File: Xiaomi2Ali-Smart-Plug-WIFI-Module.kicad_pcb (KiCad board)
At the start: 2 copper layers, 18.6 x 45 mm, 9 parts, among them J1 Conn_01x07, J2 Conn_01x03, SW1 SW_Push

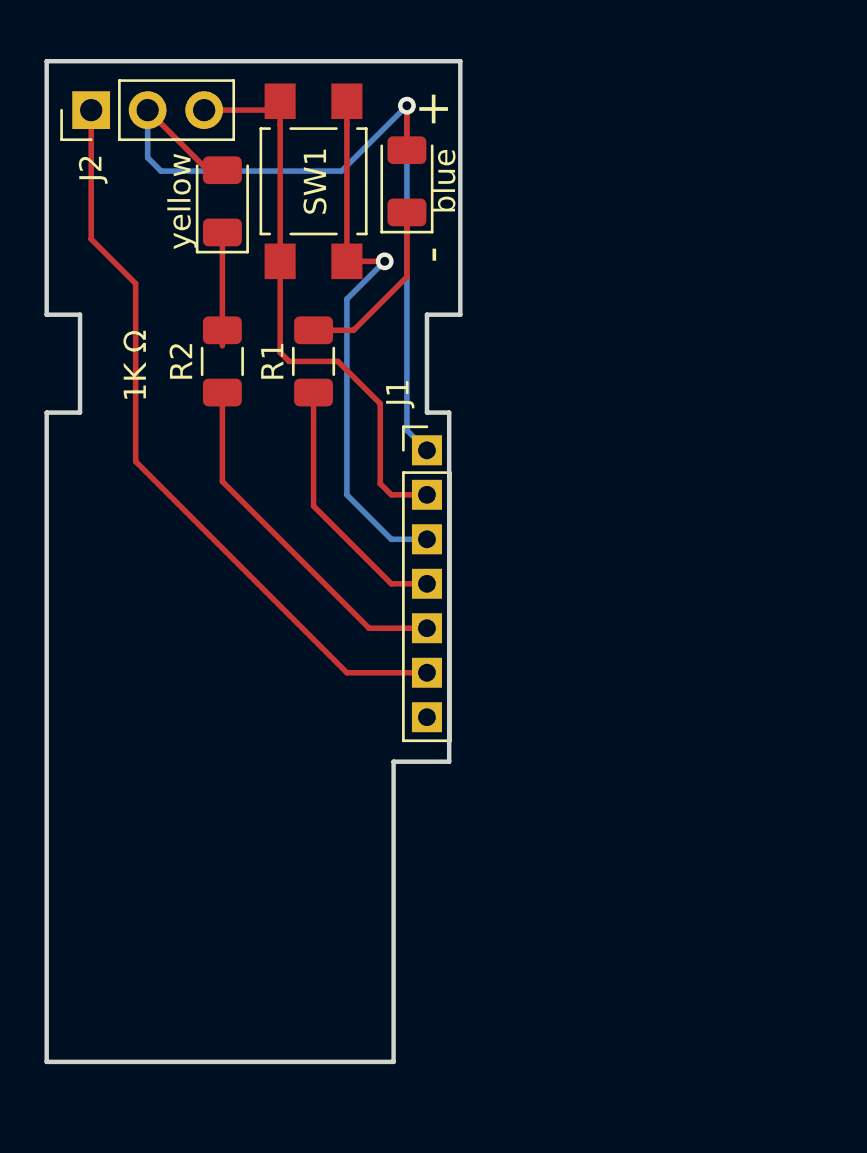
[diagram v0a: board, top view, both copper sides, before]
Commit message: Updated: 2019-02-18 18:36:52
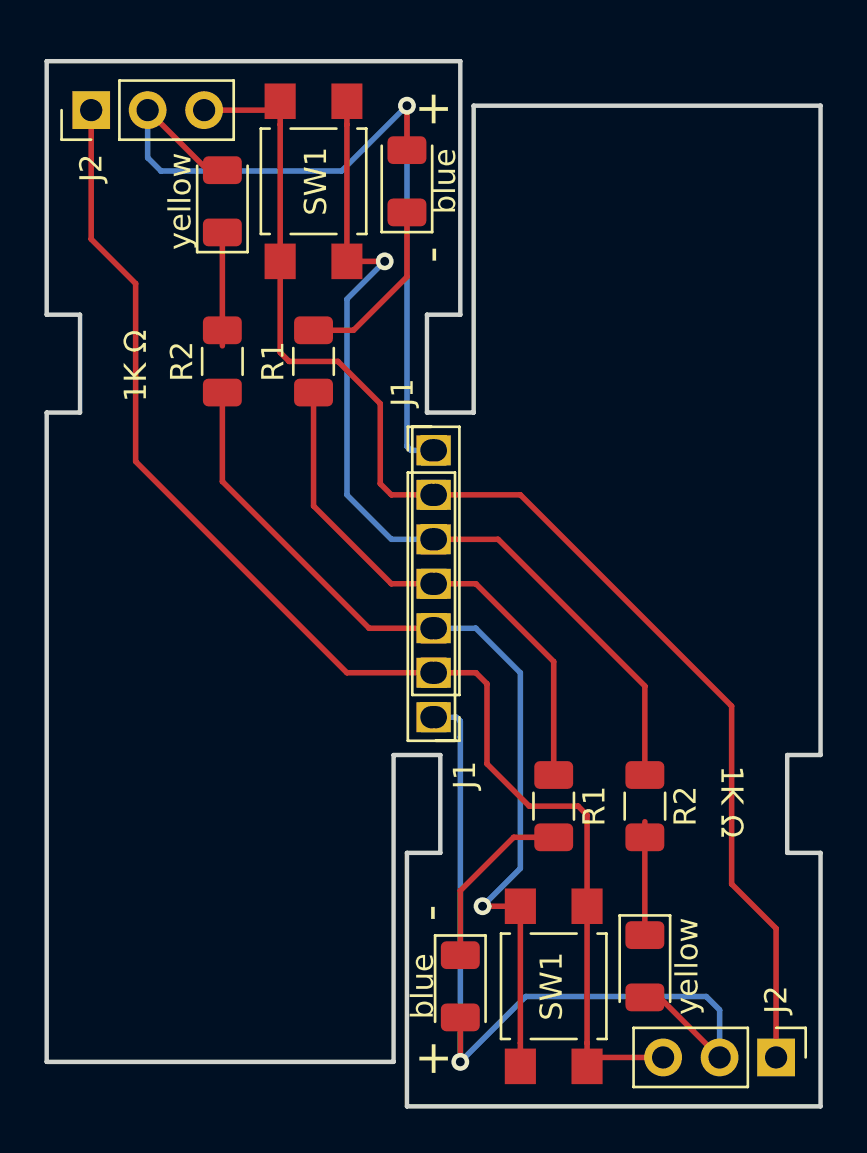
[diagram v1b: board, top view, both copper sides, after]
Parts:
- removed the J1 at (143.1, 87.5)
- added J1: Conn_01x07, Connector_PinHeader_2.00mm:PinHeader_1x07_P2.00mm_Vertical, F.Cu at (143.3, 87.5)
- added J1: Conn_01x07, Connector_PinHeader_2.00mm:PinHeader_1x07_P2.00mm_Vertical, F.Cu at (143.5, 99.5)
- added J2: Conn_01x03, Connector_PinHeader_2.54mm:PinHeader_1x03_P2.54mm_Vertical, F.Cu at (158.8, 114.8)
- added R1: 1K, Resistor_SMD:R_1206_3216Metric, F.Cu at (148.8, 103.5)
- added R2: 1K, Resistor_SMD:R_1206_3216Metric, F.Cu at (152.9, 103.5)
- added REF**: OSHW-Logo2_9.8x8mm_SilkScreen, Symbol:OSHW-Logo2_9.8x8mm_SilkScreen, B.Cu at (152.8, 86.2)
- added REF**: KiCad-Logo2_6mm_SilkScreen, Symbol:KiCad-Logo2_6mm_SilkScreen, B.Cu at (152.8, 77.0)
- added SW1: SW_Push, Button_Switch_SMD:SW_SPST_TL3305A, F.Cu at (148.8, 111.6)
- added blue: LED_blue, LED_SMD:LED_1206_3216Metric, F.Cu at (144.6, 111.6)
- added yellow: LED_yellow, LED_SMD:LED_1206_3216Metric, F.Cu at (152.9, 110.7)
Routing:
- net (no net): track 0.00 -> 163.9 mm, vias 0 -> 2
- net VCC: track 37.0 -> 38.2 mm
- net Net-(J1-Pad6): track 33.2 -> 33.9 mm
- net Net-(J1-Pad5): track 15.5 -> 16.1 mm
- net Net-(J1-Pad4): track 11.2 -> 11.8 mm
- net Net-(J1-Pad3): track 24.3 -> 24.9 mm
- net GND: track 25.8 -> 26.4 mm
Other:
- board size 18.6 x 45 mm -> 34.8 x 47 mm

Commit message: Updated: 2019-02-20 00:25:07
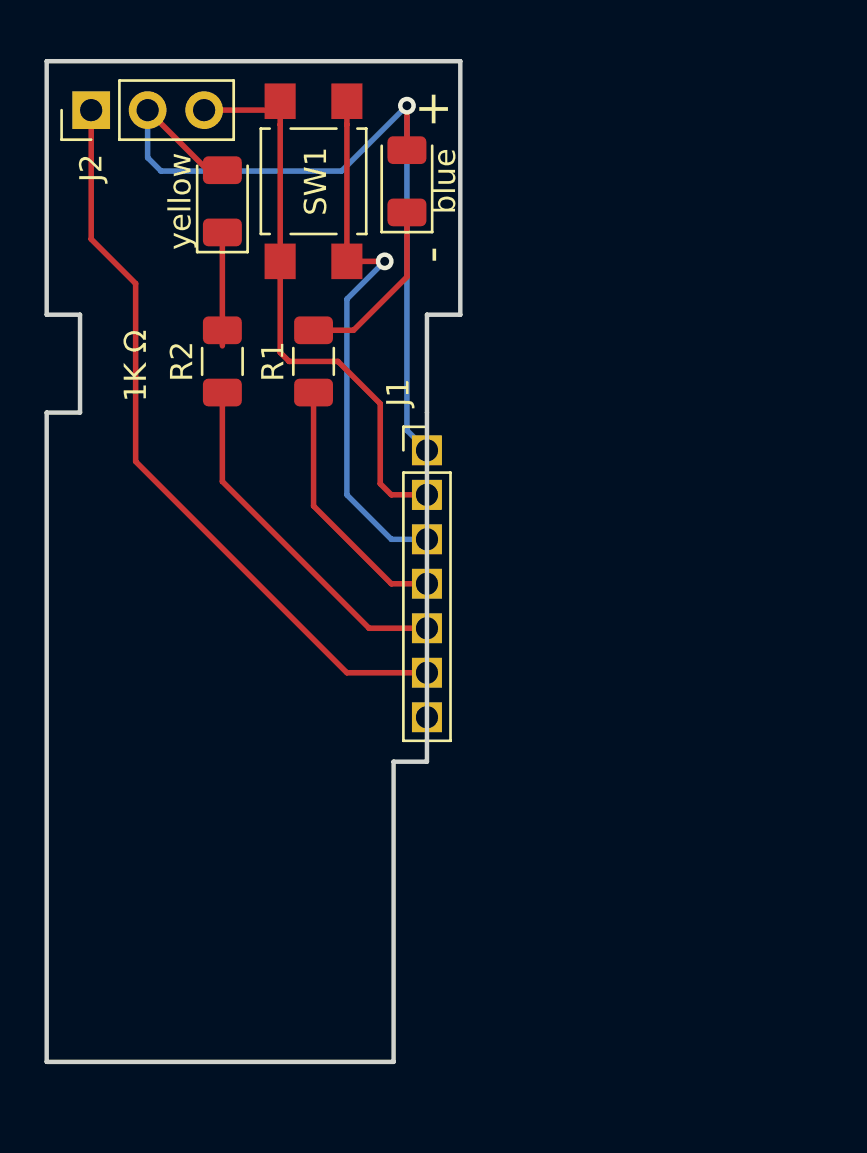
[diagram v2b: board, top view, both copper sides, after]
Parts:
- removed the J1 at (143.3, 87.5)
- removed the J1 at (143.5, 99.5)
- removed the J2 at (158.8, 114.8)
- removed the R1 at (148.8, 103.5)
- removed the R2 at (152.9, 103.5)
- removed the REF** at (152.8, 86.2)
- removed the REF** at (152.8, 77.0)
- removed the SW1 at (148.8, 111.6)
- removed the blue at (144.6, 111.6)
- removed the yellow at (152.9, 110.7)
- added J1: Conn_01x07, Connector_PinHeader_2.00mm:PinHeader_1x07_P2.00mm_Vertical, F.Cu at (143.1, 87.5)
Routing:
- net (no net): track 163.9 -> 0.00 mm, vias 2 -> 0
- net VCC: track 38.2 -> 37.0 mm
- net Net-(J1-Pad6): track 33.9 -> 33.2 mm
- net Net-(J1-Pad5): track 16.1 -> 15.5 mm
- net Net-(J1-Pad4): track 11.8 -> 11.2 mm
- net Net-(J1-Pad3): track 24.9 -> 24.3 mm
- net GND: track 26.4 -> 25.8 mm
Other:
- board size 34.8 x 47 mm -> 18.6 x 45 mm

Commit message: Updated: 2019-02-20 16:21:37
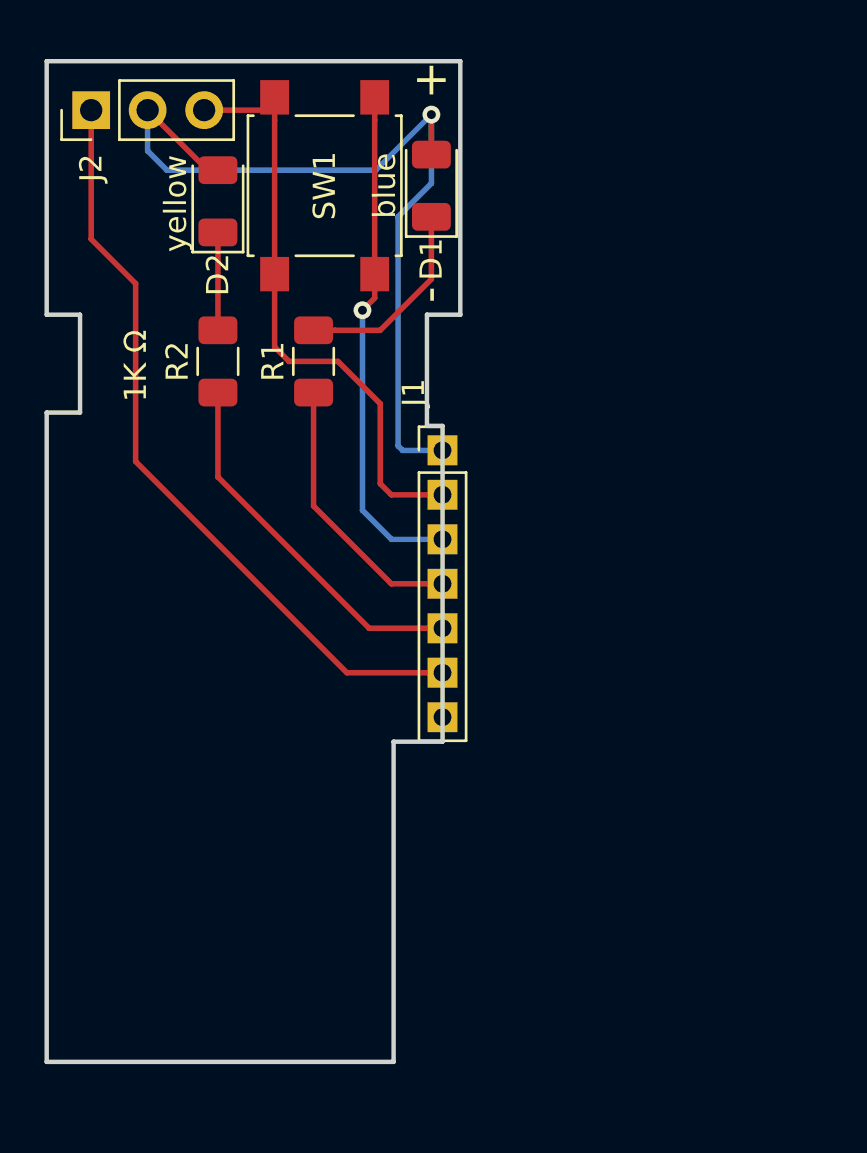
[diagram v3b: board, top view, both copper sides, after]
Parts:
- SW1: footprint Button_Switch_SMD:SW_SPST_TL3305A -> Button_Switch_SMD:SW_SPST_B3S-1000
- moved D1 1.12 mm to (143.3, 75.6)
- moved J1 0.70 mm to (143.8, 87.5)
- moved SW1 0.54 mm to (138.5, 75.6)
- moved D2 0.20 mm to (133.7, 76.3)
- moved R2 0.20 mm to (133.7, 83.5)
- renumbered blue to D1, yellow to D2
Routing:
- net VCC: track 37.0 -> 39.4 mm
- net Net-(J1-Pad3): track 24.3 -> 22.5 mm
- net GND: track 25.8 -> 27.2 mm
- net Net-(D1-Pad1): track 8.09 -> 9.05 mm
- net Net-(J1-Pad5): track 15.5 -> 16.3 mm
- net Net-(D2-Pad1): track 5.10 -> 4.40 mm
- net Net-(J1-Pad6): track 33.2 -> 33.9 mm
- net Net-(J1-Pad4): track 11.2 -> 11.9 mm
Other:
- outline, holes or cut-outs redrawn
- board text added: "blue"
- board text added: "yellow"

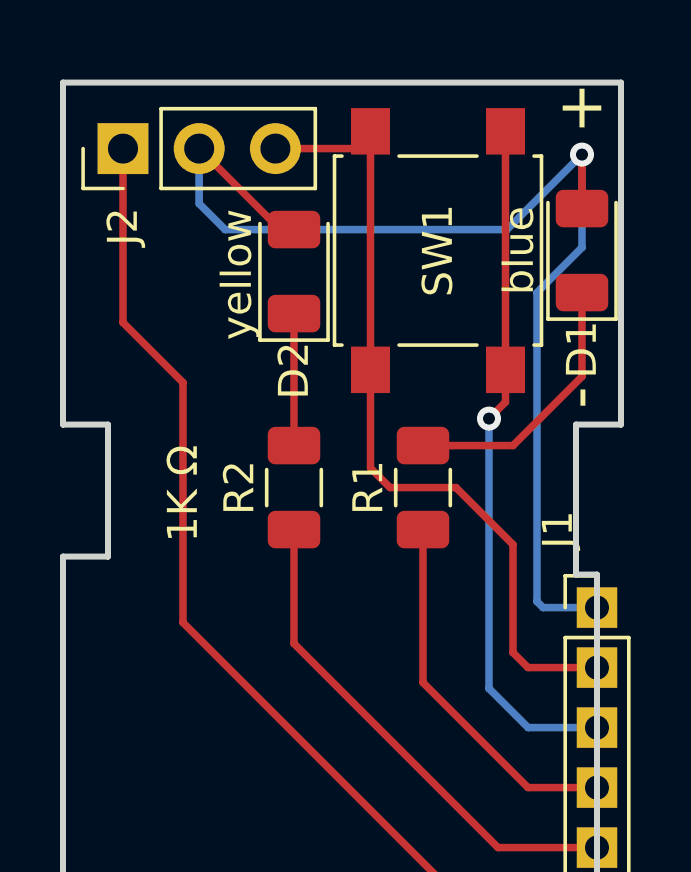
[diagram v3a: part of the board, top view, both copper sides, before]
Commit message: Updated: 2019-02-22 14:43:09
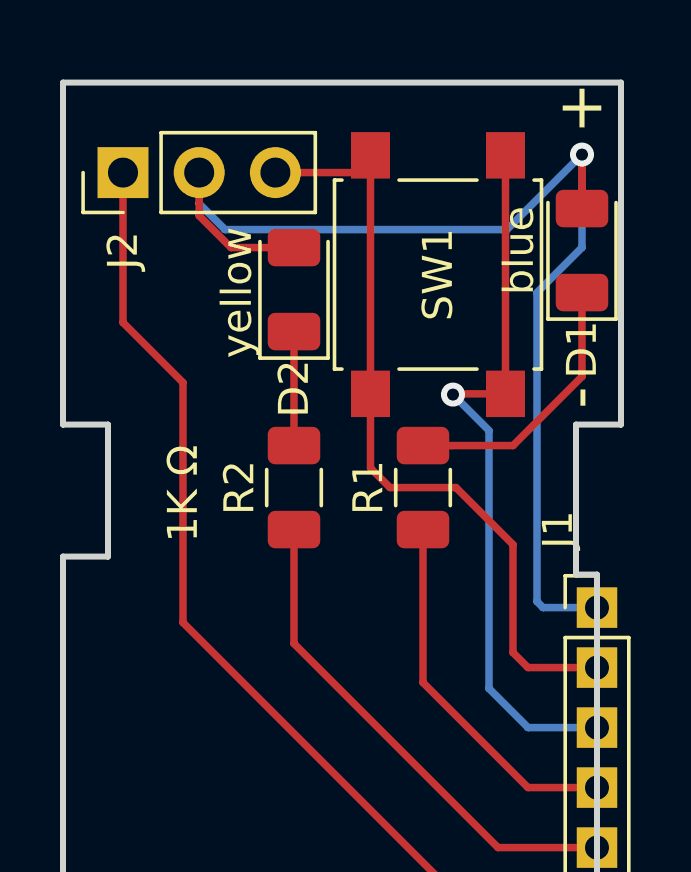
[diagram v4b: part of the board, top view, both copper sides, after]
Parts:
- moved SW1 0.80 mm to (138.5, 76.4)
- moved J2 0.80 mm to (128.0, 73.0)
- moved D2 0.60 mm to (133.7, 76.9)
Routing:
- net Net-(J1-Pad3): track 22.5 -> 23.7 mm
- net Net-(J1-Pad6): track 33.9 -> 33.1 mm
- net GND: track 27.2 -> 26.4 mm
- net Net-(D2-Pad1): track 4.40 -> 3.80 mm
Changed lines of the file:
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@@
     (thickness 1.6)
     (drawings 21)
-    (tracks 50)
+    (tracks 51)
     (zones 0)
     (modules 9)
@@
   )
   (module Button_Switch_SMD:SW_SPST_B3S-1000 (layer F.Cu)
-    (at 138.5 75.6 90)
+    (at 138.5 76.4 90)
     (descr "Surface Mount Tactile Switch for High-Density Packaging")
     (tags "Tactile Switch")
@@
   )
   (module LED_SMD:LED_1206_3216Metric (layer F.Cu)
-    (at 133.7 76.3 90)
+    (at 133.7 76.9 90)
     (descr "LED SMD 1206 (3216 Metric), square (rectangular) end terminal, IPC_7351 nominal, (Body size source: http://www.tortai-tech.com/upload/download/2011102023233369053.pdf), generated with kicad-footprint-generator")
     (tags diode)
@@
   )
   (module Connector_PinHeader_2.54mm:PinHeader_1x03_P2.54mm_Vertical (layer F.Cu)
-    (at 128 72.2 90)
+    (at 128 73 90)
     (descr "Through hole straight pin header, 1x03, 2.54mm pitch, single row")
     (tags "Through hole pin header THT 1x03 2.54mm single row")
@@
       (xy -3.43224 -2.584467) (xy -3.324904 -2.572722) (xy -3.231114 -2.584505)) (layer B.SilkS) (width 0.01))
   )
-  (gr_text yellow (at 131.8 76.4 90) (layer F.SilkS)
+  (gr_text yellow (at 131.8 77 90) (layer F.SilkS)
     (effects (font (size 1 1) (thickness 0.15)))
   )
@@
   (gr_line (start 144.6 70) (end 144.6 81.4) (layer Edge.Cuts) (width 0.2))
   (gr_line (start 126 70) (end 144.6 70) (layer Edge.Cuts) (width 0.2))
-  (via (at 140.2 81.2) (size 0.8) (drill 0.4) (layers F.Cu B.Cu) (net 5))
   (segment (start 138.975 82.1) (end 138 82.1) (width 0.25) (layer F.Cu) (net 1))
   (segment (start 141 82.1) (end 138.975 82.1) (width 0.25) (layer F.Cu) (net 1))
   (segment (start 143.3 77) (end 143.3 79.8) (width 0.25) (layer F.Cu) (net 1))
   (segment (start 143.3 79.8) (end 141 82.1) (width 0.25) (layer F.Cu) (net 1))
-  (segment (start 133.24 74.9) (end 133.9 74.9) (width 0.25) (layer F.Cu) (net 2))
-  (segment (start 130.54 72.2) (end 133.24 74.9) (width 0.25) (layer F.Cu) (net 2))
   (segment (start 133.9 74.9) (end 133.9 74.9) (width 0.25) (layer F.Cu) (net 2))
   (via (at 143.3 72.4) (size 0.8) (drill 0.4) (layers F.Cu B.Cu) (net 2))
@@
   (segment (start 142 87.5) (end 143.37499 87.5) (width 0.25) (layer B.Cu) (net 2))
   (segment (start 143.3 72.4) (end 143.3 74.2) (width 0.25) (layer F.Cu) (net 2))
-  (segment (start 140.8 74.9) (end 143.3 72.4) (width 0.25) (layer B.Cu) (net 2))
-  (segment (start 131.4 74.9) (end 140.8 74.9) (width 0.25) (layer B.Cu) (net 2))
-  (segment (start 130.54 72.2) (end 130.54 74.04) (width 0.25) (layer B.Cu) (net 2))
-  (segment (start 130.54 74.04) (end 131.4 74.9) (width 0.25) (layer B.Cu) (net 2))
   (segment (start 141.8 87.3) (end 141.8 77) (width 0.25) (layer B.Cu) (net 2))
   (segment (start 143.3 75.5) (end 143.3 72.4) (width 0.25) (layer B.Cu) (net 2))
   (segment (start 141.8 77) (end 143.3 75.5) (width 0.25) (layer B.Cu) (net 2))
-  (segment (start 133.7 82.1) (end 133.7 77.7) (width 0.25) (layer F.Cu) (net 3))
+  (segment (start 130.54 74.04) (end 130.54 73) (width 0.25) (layer B.Cu) (net 2))
+  (segment (start 131.4 74.9) (end 130.54 74.04) (width 0.25) (layer B.Cu) (net 2))
+  (segment (start 143.3 72.4) (end 140.8 74.9) (width 0.25) (layer B.Cu) (net 2))
+  (segment (start 140.8 74.9) (end 131.4 74.9) (width 0.25) (layer B.Cu) (net 2))
+  (segment (start 131.6 75.5) (end 133.7 75.5) (width 0.25) (layer F.Cu) (net 2))
+  (segment (start 130.54 73) (end 130.54 74.44) (width 0.25) (layer F.Cu) (net 2))
+  (segment (start 130.54 74.44) (end 131.6 75.5) (width 0.25) (layer F.Cu) (net 2))
+  (segment (start 133.7 78.3) (end 133.7 82.1) (width 0.25) (layer F.Cu) (net 3))
   (segment (start 136.1 72.2) (end 136.5 71.8) (width 0.25) (layer F.Cu) (net 4))
   (segment (start 136.9 83.5) (end 139.1 83.5) (width 0.25) (layer F.Cu) (net 4))
@@
   (segment (start 141 85.4) (end 141 89) (width 0.25) (layer F.Cu) (net 4))
   (segment (start 141 89) (end 141.5 89.5) (width 0.25) (layer F.Cu) (net 4))
-  (segment (start 135.675 72.2) (end 136.25 71.625) (width 0.25) (layer F.Cu) (net 4))
-  (segment (start 133.08 72.2) (end 135.675 72.2) (width 0.25) (layer F.Cu) (net 4))
-  (segment (start 136.25 72.65) (end 136.25 79.575) (width 0.25) (layer F.Cu) (net 4))
-  (segment (start 136.25 71.625) (end 136.25 72.65) (width 0.25) (layer F.Cu) (net 4))
   (segment (start 136.25 82.85) (end 136.9 83.5) (width 0.25) (layer F.Cu) (net 4))
-  (segment (start 136.25 79.575) (end 136.25 82.85) (width 0.25) (layer F.Cu) (net 4))
   (segment (start 141.5 89.5) (end 143.37499 89.5) (width 0.25) (layer F.Cu) (net 4))
-  (segment (start 140.75 72.65) (end 140.75 79.575) (width 0.25) (layer F.Cu) (net 5))
-  (segment (start 140.75 71.625) (end 140.75 72.65) (width 0.25) (layer F.Cu) (net 5))
-  (segment (start 140.2 81.2) (end 140.2 90.2) (width 0.25) (layer B.Cu) (net 5))
+  (segment (start 135.675 73) (end 136.25 72.425) (width 0.25) (layer F.Cu) (net 4))
+  (segment (start 133.08 73) (end 135.675 73) (width 0.25) (layer F.Cu) (net 4))
+  (segment (start 136.25 72.425) (end 136.25 80.375) (width 0.25) (layer F.Cu) (net 4))
+  (segment (start 136.25 80.375) (end 136.25 82.85) (width 0.25) (layer F.Cu) (net 4))
+  (via (at 139 80.4) (size 0.8) (drill 0.4) (layers F.Cu B.Cu) (net 5))
   (segment (start 140.2 90.2) (end 141.5 91.5) (width 0.25) (layer B.Cu) (net 5))
-  (segment (start 140.75 80.65) (end 140.2 81.2) (width 0.25) (layer F.Cu) (net 5))
-  (segment (start 140.75 79.575) (end 140.75 80.65) (width 0.25) (layer F.Cu) (net 5))
   (segment (start 141.5 91.5) (end 143.37499 91.5) (width 0.25) (layer B.Cu) (net 5))
+  (segment (start 140.75 73.45) (end 140.75 80.375) (width 0.25) (layer F.Cu) (net 5))
+  (segment (start 140.75 72.425) (end 140.75 73.45) (width 0.25) (layer F.Cu) (net 5))
+  (segment (start 139.025 80.375) (end 139 80.4) (width 0.25) (layer F.Cu) (net 5))
+  (segment (start 140.75 80.375) (end 139.025 80.375) (width 0.25) (layer F.Cu) (net 5))
+  (segment (start 139 80.4) (end 140.2 81.6) (width 0.25) (layer B.Cu) (net 5))
+  (segment (start 140.2 81.6) (end 140.2 90.2) (width 0.25) (layer B.Cu) (net 5))
   (segment (start 138 84.9) (end 138 90) (width 0.25) (layer F.Cu) (net 6))
   (segment (start 138 90) (end 141.5 93.5) (width 0.25) (layer F.Cu) (net 6))
@@
   (segment (start 130 88) (end 139.5 97.5) (width 0.25) (layer F.Cu) (net 8))
   (segment (start 130 80) (end 130 88) (width 0.25) (layer F.Cu) (net 8))
-  (segment (start 128 72.2) (end 128 78) (width 0.25) (layer F.Cu) (net 8))
   (segment (start 128 78) (end 130 80) (width 0.25) (layer F.Cu) (net 8))
   (segment (start 139.5 97.5) (end 143.37499 97.5) (width 0.25) (layer F.Cu) (net 8))
+  (segment (start 128 73) (end 128 78) (width 0.25) (layer F.Cu) (net 8))
 )
